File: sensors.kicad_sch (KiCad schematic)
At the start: 8 parts, among them J4 Conn_01x05_Pin, U3 MMC5983MA, U4 BMI088, U9 MCP23009-E/MG

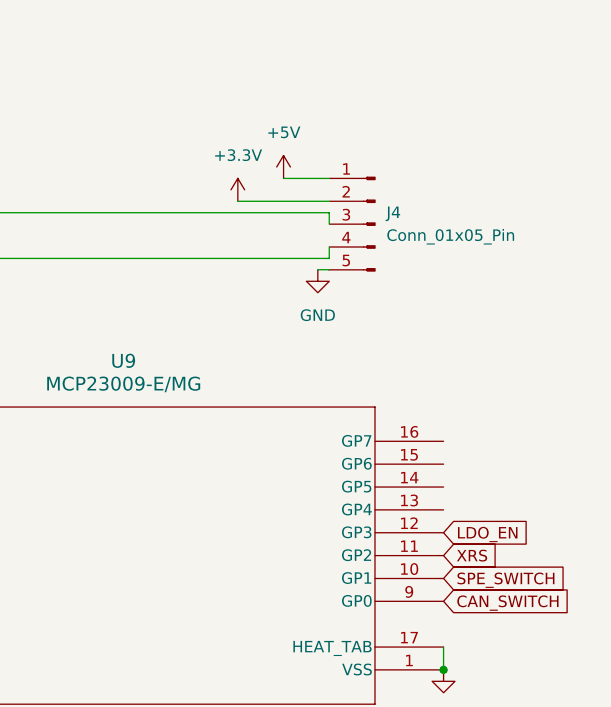
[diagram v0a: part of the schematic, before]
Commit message: save before sdram redesign
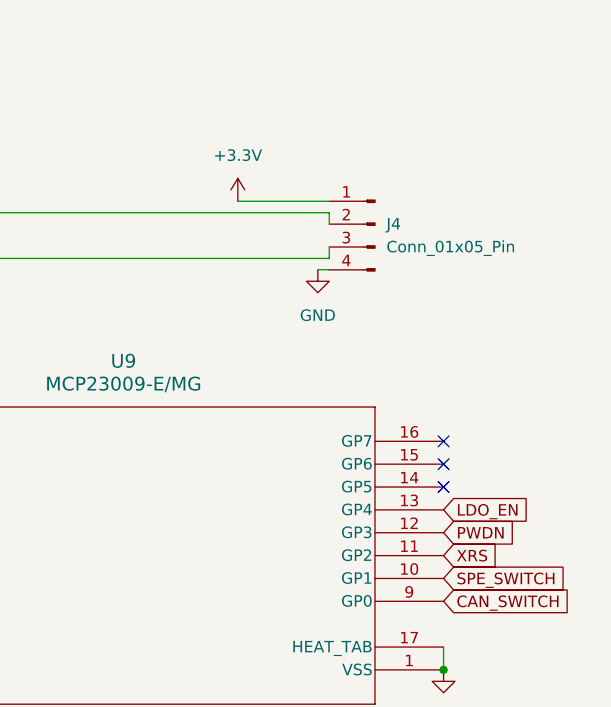
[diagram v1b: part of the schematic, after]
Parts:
- C50, C51: footprint Capacitor_SMD:C_0402_1005Metric -> Capacitor_SMD:C_0201_0603Metric
- J4: symbol Connector:Conn_01x05_Pin -> Connector:Conn_01x04_Pin
- U3: footprint MMC5983MA:PQFN50P300X300X100-16N -> footprints:PQFN50P300X300X100-16N
- U4: footprint BMI088:PQFN50P450X300X100-16N -> footprints:PQFN50P450X300X100-16N
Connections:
- net +5V is gone; now on net +3.3V: J4.1 (Pin_1)
- net +3.3V: no longer J4.2 (Pin_2)
- net GND: now also J4.4 (Pin_4); no longer J4.5 (Pin_5)
- net LDO_EN: now also U9.13 (GP4); no longer U9.12 (GP3)
- net LPI2C1_SCL: now also J4.3 (Pin_3); no longer J4.4 (Pin_4)
- net LPI2C1_SDA: now also J4.2 (Pin_2); no longer J4.3 (Pin_3)
- new net PWDN: U9.12 (GP3)
- no-connect marks 10 -> 13
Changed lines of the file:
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@@
+	)
+	(no_connect
+		(at 260.35 74.93)
+	)
+	(no_connect
+		(at 260.35 77.47)
 	)
 	(no_connect
@@
 	)
 	(no_connect
+		(at 260.35 72.39)
+	)
+	(no_connect
 		(at 127 90.17)
 	)
@@
 		(pts
 			(xy 50.8 46.99) (xy 121.92 46.99)
-		)
-		(stroke
-			(width 0)
-			(type default)
-		)
-	)
-	(wire
-		(pts
-			(xy 242.57 43.18) (xy 247.65 43.18)
 		)
 		(stroke
@@
 		)
 	)
-	(global_label "LDO_EN"
+	(global_label "XRS"
 		(shape input)
-		(at 260.35 82.55 0)
+		(at 260.35 85.09 0)
 		(fields_autoplaced yes)
 		(effects
@@
 		)
 		(property "Intersheetrefs" "${INTERSHEET_REFS}"
-			(at 270.4109 82.55 0)
+			(at 267.0242 85.09 0)
+			(effects
+				(font
+					(size 1.27 1.27)
+				)
+				(justify left)
+				(hide yes)
+			)
+		)
+	)
+	(global_label "PWDN"
+		(shape input)
+		(at 260.35 82.55 0)
+		(fields_autoplaced yes)
+		(effects
+			(font
+				(size 1.27 1.27)
+			)
+			(justify left)
+		)
+		(property "Intersheetrefs" "${INTERSHEET_REFS}"
+			(at 268.6571 82.55 0)
+			(effects
+				(font
+					(size 1.27 1.27)
+				)
+				(justify left)
+				(hide yes)
+			)
+		)
+	)
+	(global_label "LDO_EN"
+		(shape input)
+		(at 260.35 80.01 0)
+		(fields_autoplaced yes)
+		(effects
+			(font
+				(size 1.27 1.27)
+			)
+			(justify left)
+		)
+		(property "Intersheetrefs" "${INTERSHEET_REFS}"
+			(at 270.4109 80.01 0)
 			(effects
 				(font
@@
 				)
 				(justify right)
-				(hide yes)
-			)
-		)
-	)
-	(global_label "XRS"
-		(shape input)
-		(at 260.35 85.09 0)
-		(fields_autoplaced yes)
-		(effects
-			(font
-				(size 1.27 1.27)
-			)
-			(justify left)
-		)
-		(property "Intersheetrefs" "${INTERSHEET_REFS}"
-			(at 267.0242 85.09 0)
-			(effects
-				(font
-					(size 1.27 1.27)
-				)
-				(justify left)
 				(hide yes)
 			)
@@
 			)
 		)
+		(property "Flight" ""
+			(at 189.23 73.66 0)
+			(effects
+				(font
+					(size 1.27 1.27)
+				)
+				(hide yes)
+			)
+		)
+		(property "Proto" ""
+			(at 189.23 73.66 0)
+			(effects
+				(font
+					(size 1.27 1.27)
+				)
+				(hide yes)
+			)
+		)
 		(pin "6"
 		)
@@
 			)
 		)
-		(property "Footprint" "Capacitor_SMD:C_0402_1005Metric"
+		(property "Footprint" "Capacitor_SMD:C_0201_0603Metric"
 			(at 54.61 88.9 0)
 			(effects
@@
 		)
 		(property "Description" "Unpolarized capacitor, small symbol"
+			(at 54.61 88.9 0)
+			(effects
+				(font
+					(size 1.27 1.27)
+				)
+				(hide yes)
+			)
+		)
+		(property "Flight" ""
+			(at 54.61 88.9 0)
+			(effects
+				(font
+					(size 1.27 1.27)
+				)
+				(hide yes)
+			)
+		)
+		(property "Proto" ""
 			(at 54.61 88.9 0)
 			(effects
@@
 			)
 		)
+		(property "Flight" ""
+			(at 35.56 39.37 0)
+			(effects
+				(font
+					(size 1.27 1.27)
+				)
+				(hide yes)
+			)
+		)
+		(property "Proto" ""
+			(at 35.56 39.37 0)
+			(effects
+				(font
+					(size 1.27 1.27)
+				)
+				(hide yes)
+			)
+		)
 		(pin "1"
 		)
@@
 			)
 		)
-		(property "Footprint" "MMC5983MA:PQFN50P300X300X100-16N"
+		(property "Footprint" "footprints:PQFN50P300X300X100-16N"
 			(at 78.74 81.28 0)
 			(effects
@@
 				)
 				(justify bottom)
+				(hide yes)
+			)
+		)
+		(property "Flight" ""
+			(at 78.74 81.28 0)
+			(effects
+				(font
+					(size 1.27 1.27)
+				)
+				(hide yes)
+			)
+		)
+		(property "Proto" ""
+			(at 78.74 81.28 0)
+			(effects
+				(font
+					(size 1.27 1.27)
+				)
 				(hide yes)
 			)
@@
 			)
 		)
-		(property "Footprint" "BMI088:PQFN50P450X300X100-16N"
+		(property "Footprint" "footprints:PQFN50P450X300X100-16N"
 			(at 144.78 92.71 0)
 			(effects
@@
 				)
 				(justify bottom)
+				(hide yes)
+			)
+		)
+		(property "Flight" ""
+			(at 144.78 92.71 0)
+			(effects
+				(font
+					(size 1.27 1.27)
+				)
+				(hide yes)
+			)
+		)
+		(property "Proto" ""
+			(at 144.78 92.71 0)
+			(effects
+				(font
+					(size 1.27 1.27)
+				)
 				(hide yes)
 			)
@@
 			)
 		)
+		(property "Flight" ""
+			(at 44.45 39.37 0)
+			(effects
+				(font
+					(size 1.27 1.27)
+				)
+				(hide yes)
+			)
+		)
+		(property "Proto" ""
+			(at 44.45 39.37 0)
+			(effects
+				(font
+					(size 1.27 1.27)
+				)
+				(hide yes)
+			)
+		)
 		(pin "1"
 		)
@@
 			)
 		)
-		(property "Footprint" "Capacitor_SMD:C_0402_1005Metric"
+		(property "Footprint" "Capacitor_SMD:C_0201_0603Metric"
 			(at 113.03 71.12 0)
 			(effects
@@
 		)
 		(property "Description" "Unpolarized capacitor, small symbol"
+			(at 113.03 71.12 0)
+			(effects
+				(font
+					(size 1.27 1.27)
+				)
+				(hide yes)
+			)
+		)
+		(property "Flight" ""
+			(at 113.03 71.12 0)
+			(effects
+				(font
+					(size 1.27 1.27)
+				)
+				(hide yes)
+			)
+		)
+		(property "Proto" ""
 			(at 113.03 71.12 0)
 			(effects
@@
 	)
 	(symbol
-		(lib_id "Connector:Conn_01x05_Pin")
+		(lib_id "Connector:Conn_01x04_Pin")
 		(at 252.73 48.26 0)
 		(mirror y)
@@
 		(fields_autoplaced yes)
 		(property "Reference" "J4"
-			(at 254 46.9899 0)
+			(at 254 48.2599 0)
 			(effects
 				(font
@@
 		)
 		(property "Value" "Conn_01x05_Pin"
-			(at 254 49.5299 0)
+			(at 254 50.7999 0)
 			(effects
 				(font
@@
 			)
 		)
-		(property "Description" "Generic connector, single row, 01x05, script generated"
+		(property "Description" "Generic connector, single row, 01x04, script generated"
 			(at 252.73 48.26 0)
 			(effects
@@
 			)
 		)
+		(property "Flight" ""
+			(at 252.73 48.26 0)
+			(effects
+				(font
+					(size 1.27 1.27)
+				)
+				(hide yes)
+			)
+		)
+		(property "Proto" ""
+			(at 252.73 48.26 0)
+			(effects
+				(font
+					(size 1.27 1.27)
+				)
+				(hide yes)
+			)
+		)
 		(pin "3"
 		)
@@
 		)
 		(pin "1"
-		)
-		(pin "5"
 		)
 		(instances
@@
 					(unit 1)
 				)
-			)
-		)
-	)
-	(symbol
-		(lib_id "power:+5V")
-		(at 242.57 43.18 0)
-		(unit 1)
-		(exclude_from_sim no)
-		(in_bom yes)
-		(on_board yes)
-		(dnp no)
-		(fields_autoplaced yes)
-		(property "Reference" "#PWR080"
-			(at 242.57 46.99 0)
-			(effects
-				(font
-					(size 1.27 1.27)
-				)
-				(hide yes)
-			)
-		)
-		(property "Value" "+5V"
-			(at 242.57 38.1 0)
-			(effects
-				(font
-					(size 1.27 1.27)
-				)
-			)
-		)
-		(property "Footprint" ""
-			(at 242.57 43.18 0)
-			(effects
-				(font
-					(size 1.27 1.27)
-				)
-				(hide yes)
-			)
-		)
-		(property "Datasheet" ""
-			(at 242.57 43.18 0)
-			(effects
-				(font
-					(size 1.27 1.27)
-				)
-				(hide yes)
-			)
-		)
-		(property "Description" "Power symbol creates a global label with name \"+5V\""
-			(at 242.57 43.18 0)
-			(effects
-				(font
-					(size 1.27 1.27)
-				)
-				(hide yes)
-			)
-		)
-		(pin "1"
-		)
-		(instances
-			(project "RT1050"
-				(path "/dd9d031d-43a1-4442-b493-27451a14e0d9/2d6e0293-1e7f-4e64-b0be-64f8e31d184d"
-					(reference "#PWR080")
-					(unit 1)
-				)

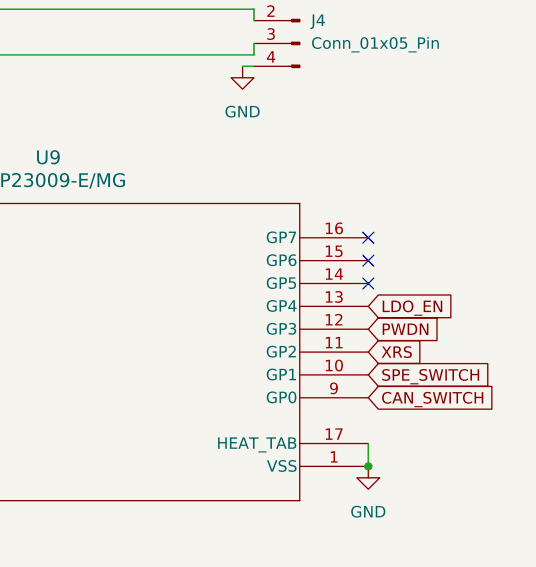
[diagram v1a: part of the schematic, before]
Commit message: SDRAM redo and finished boards
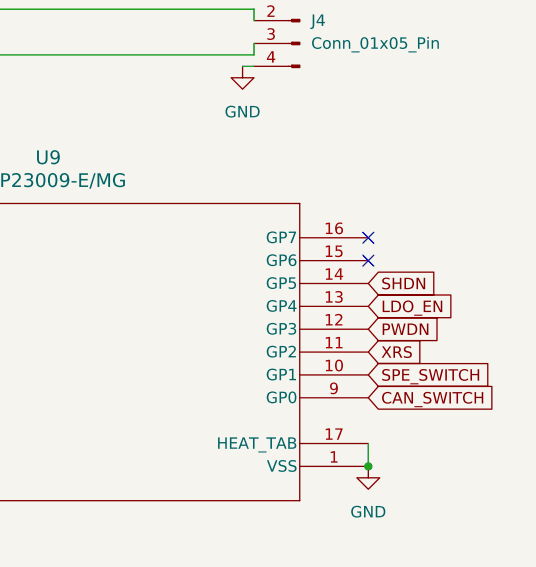
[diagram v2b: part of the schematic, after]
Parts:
- J4: footprint Connector_PinHeader_2.00mm:PinHeader_1x05_P2.00mm_Vertical -> Connector_PinHeader_2.00mm:PinHeader_1x04_P2.00mm_Vertical
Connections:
- net SHDN: now reaches U9.14 (GP5)
- no-connect marks 13 -> 12
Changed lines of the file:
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@@
-	)
-	(no_connect
-		(at 260.35 77.47)
 	)
 	(no_connect
@@
 				)
 				(justify left)
+				(hide yes)
+			)
+		)
+	)
+	(global_label "SHDN"
+		(shape input)
+		(at 260.35 77.47 0)
+		(effects
+			(font
+				(size 1.27 1.27)
+			)
+			(justify left)
+		)
+		(property "Intersheetrefs" "${INTERSHEET_REFS}"
+			(at 260.35 77.47 0)
+			(effects
+				(font
+					(size 1.27 1.27)
+				)
 				(hide yes)
 			)
@@
 			)
 		)
-		(property "Footprint" "Connector_PinHeader_2.00mm:PinHeader_1x05_P2.00mm_Vertical"
+		(property "Footprint" "Connector_PinHeader_2.00mm:PinHeader_1x04_P2.00mm_Vertical"
 			(at 252.73 48.26 0)
 			(effects
